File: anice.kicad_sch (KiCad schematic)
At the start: 7 parts, among them J1 Conn_02x20_Counter_Clockwise, J2 Micro_SD_Card_Det1, Y1 ECS-2520MV-xxx-xx

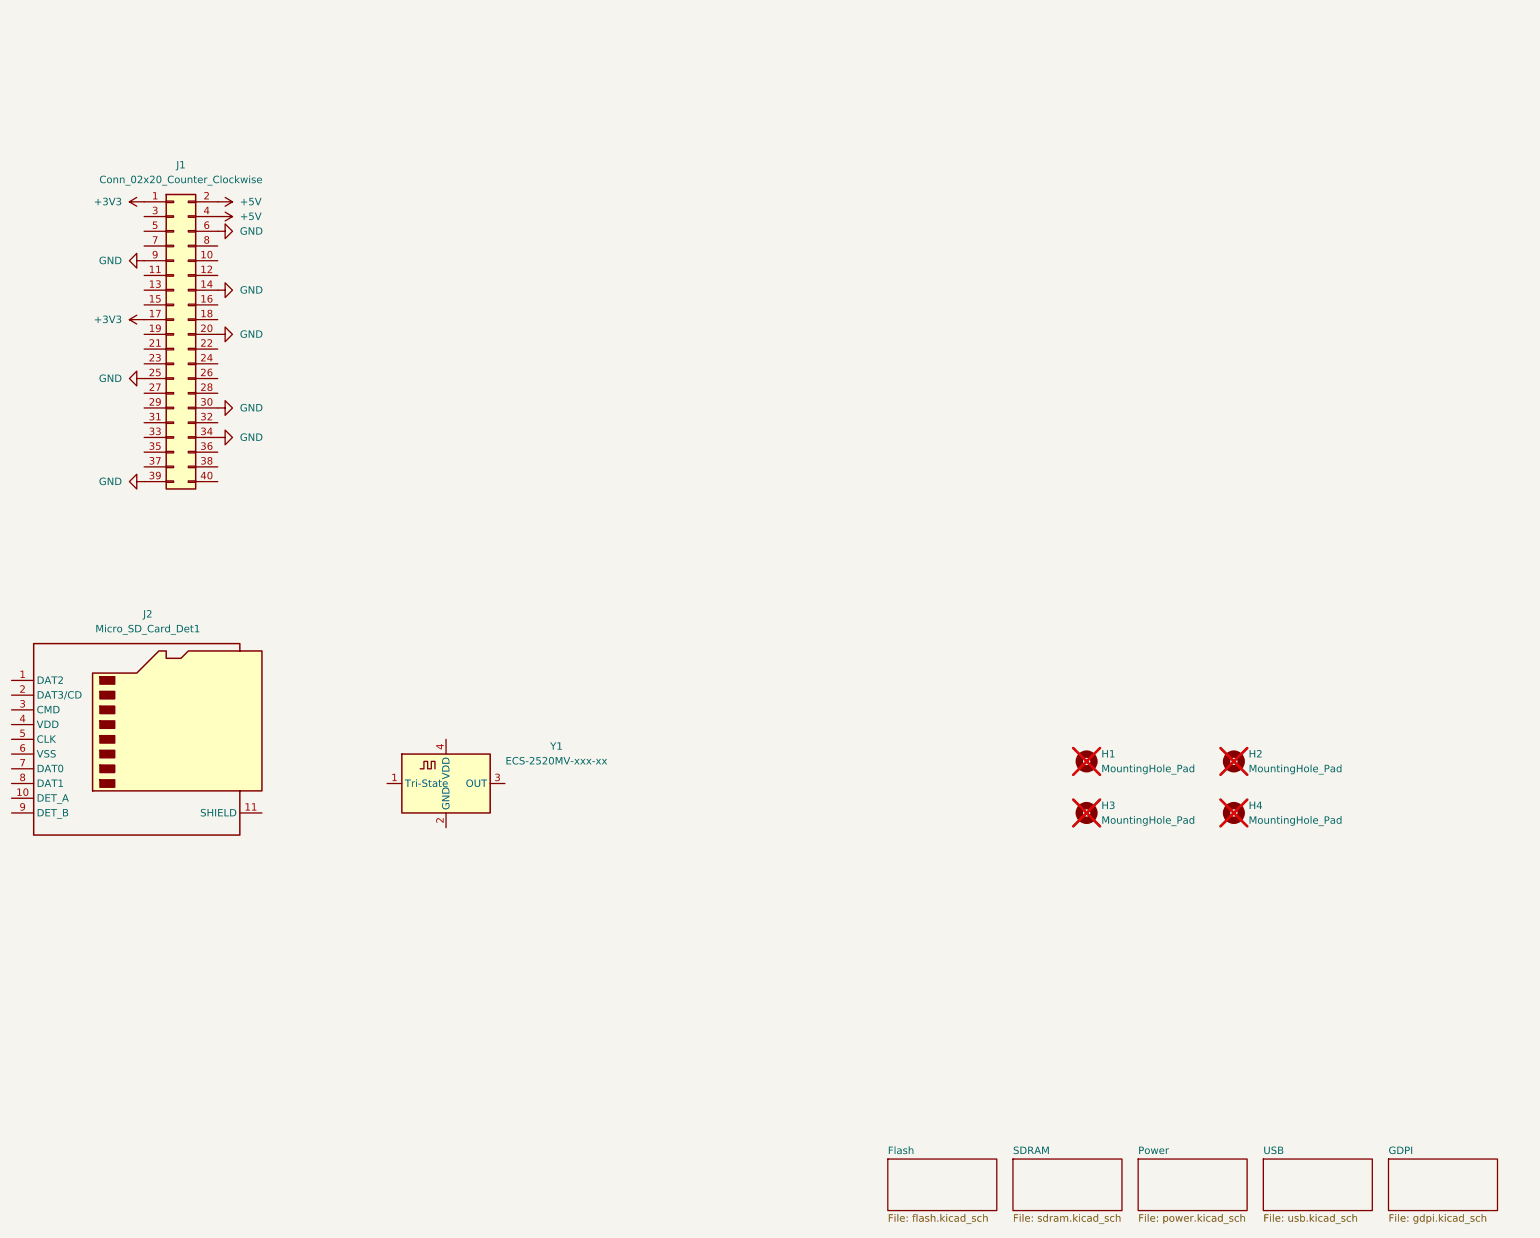
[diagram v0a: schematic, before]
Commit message: Stash
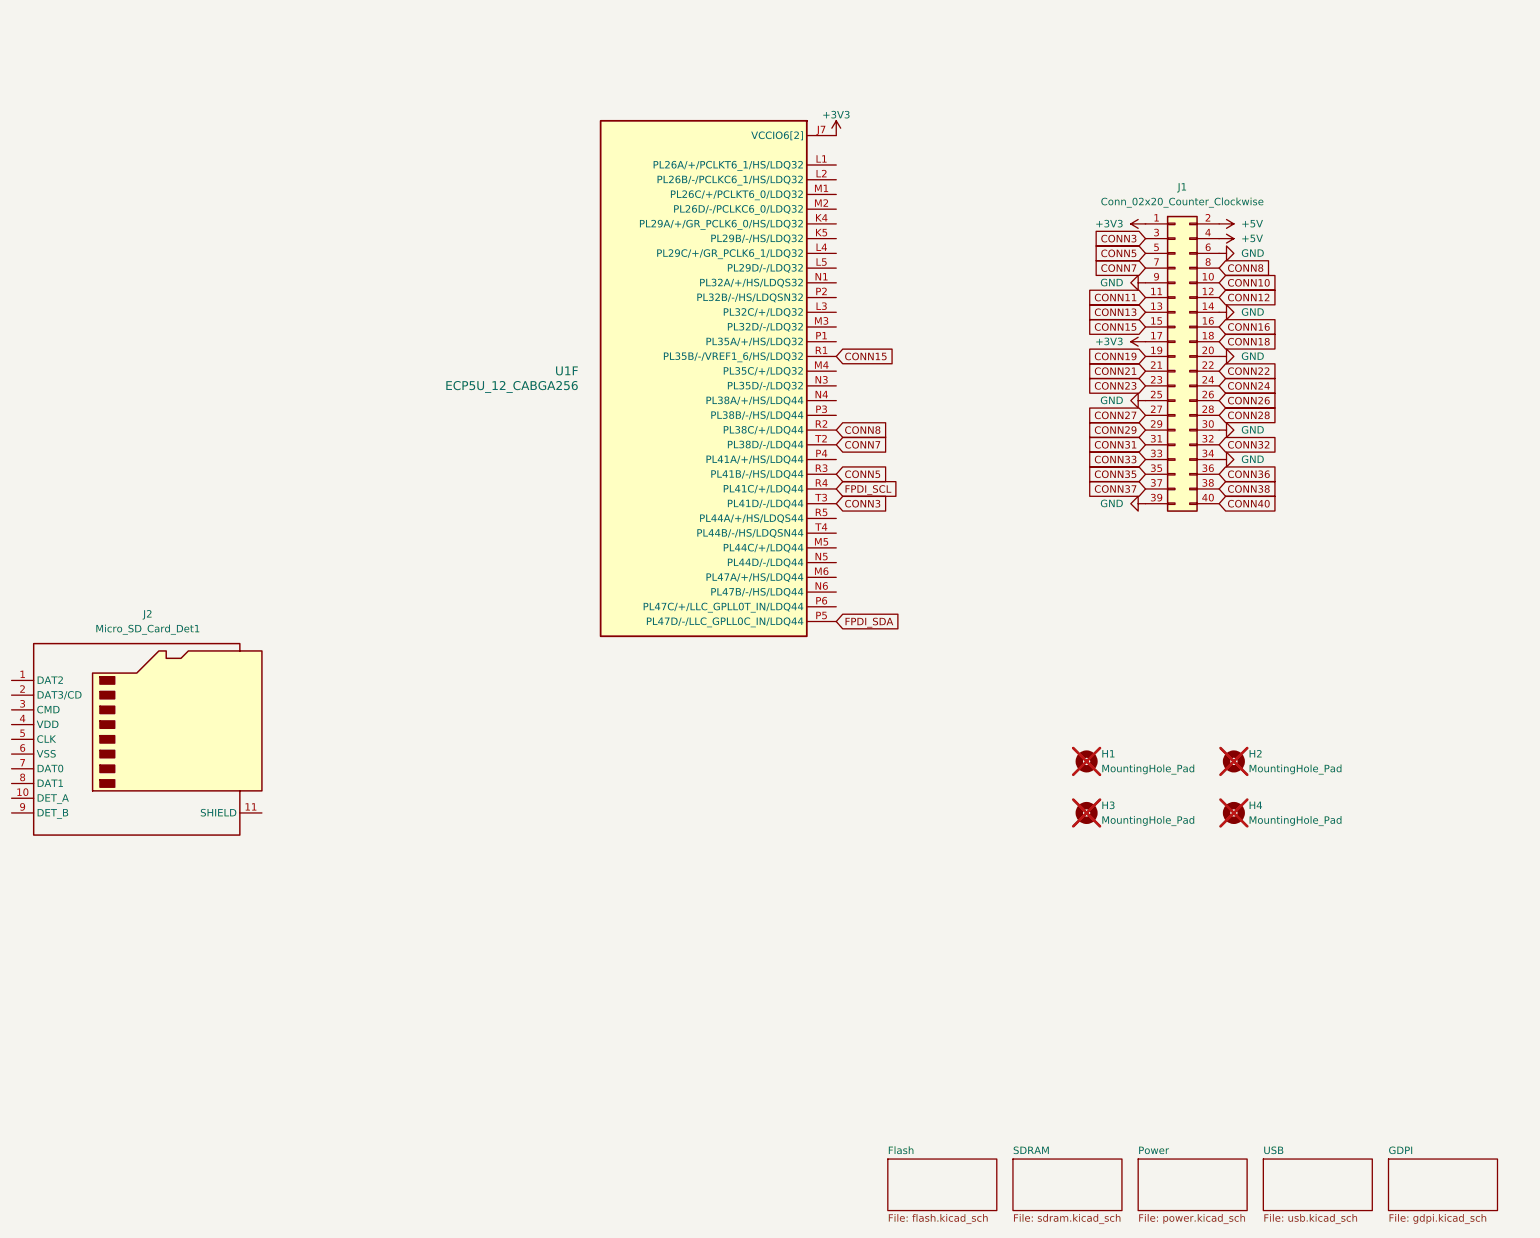
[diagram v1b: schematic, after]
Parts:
- removed Y1: ECS-2520MV-xxx-xx, Crystal:Crystal_SMD_3225-4Pin_3.2x2.5mm, symbol Oscillator:ECS-2520MV-xxx-xx
- added U1: ECP5U_12_CABGA256, Package_BGA:BGA-256_14.0x14.0mm_Layout16x16_P0.8mm_Ball0.45mm_Pad0.32mm_NSMD, symbol josh-ic:ECP5U_12_CABGA256
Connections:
- net +3V3: now also U1.J6 (VCCIO6[2]), U1.J7 (VCCIO6[2])
- net CONN10: now reaches J1.10 (Pin_10)
- net CONN11: now reaches J1.11 (Pin_11)
- net CONN12: now reaches J1.12 (Pin_12)
- net CONN13: now reaches J1.13 (Pin_13)
- net CONN15: now reaches J1.15 (Pin_15)
- net CONN15: now also U1.R1 (PL35B/-/VREF1_6/HS/LDQ32)
- net CONN16: now reaches J1.16 (Pin_16)
- net CONN18: now reaches J1.18 (Pin_18)
- net CONN19: now reaches J1.19 (Pin_19)
- net CONN21: now reaches J1.21 (Pin_21)
- net CONN22: now reaches J1.22 (Pin_22)
- net CONN23: now reaches J1.23 (Pin_23)
- net CONN24: now reaches J1.24 (Pin_24)
- net CONN26: now reaches J1.26 (Pin_26)
- net CONN27: now reaches J1.27 (Pin_27)
- net CONN28: now reaches J1.28 (Pin_28)
- net CONN29: now reaches J1.29 (Pin_29)
- net CONN3: now reaches J1.3 (Pin_3)
- net CONN3: now also U1.T3 (PL41D/-/LDQ44)
- net CONN31: now reaches J1.31 (Pin_31)
- net CONN32: now reaches J1.32 (Pin_32)
- net CONN33: now reaches J1.33 (Pin_33)
- net CONN35: now reaches J1.35 (Pin_35)
- net CONN36: now reaches J1.36 (Pin_36)
- net CONN37: now reaches J1.37 (Pin_37)
- net CONN38: now reaches J1.38 (Pin_38)
- net CONN40: now reaches J1.40 (Pin_40)
- net CONN5: now reaches J1.5 (Pin_5)
- net CONN5: now also U1.R3 (PL41B/-/HS/LDQ44)
- net CONN7: now reaches J1.7 (Pin_7)
- net CONN7: now also U1.T2 (PL38D/-/LDQ44)
- net CONN8: now reaches J1.8 (Pin_8)
- net CONN8: now also U1.R2 (PL38C/+/LDQ44)
- new net FPDI_SCL: U1.R4 (PL41C/+/LDQ44)
- new net FPDI_SDA: U1.P5 (PL47D/-/LLC_GPLL0C_IN/LDQ44)
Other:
- moved on the sheet: J1

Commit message: Rev 1
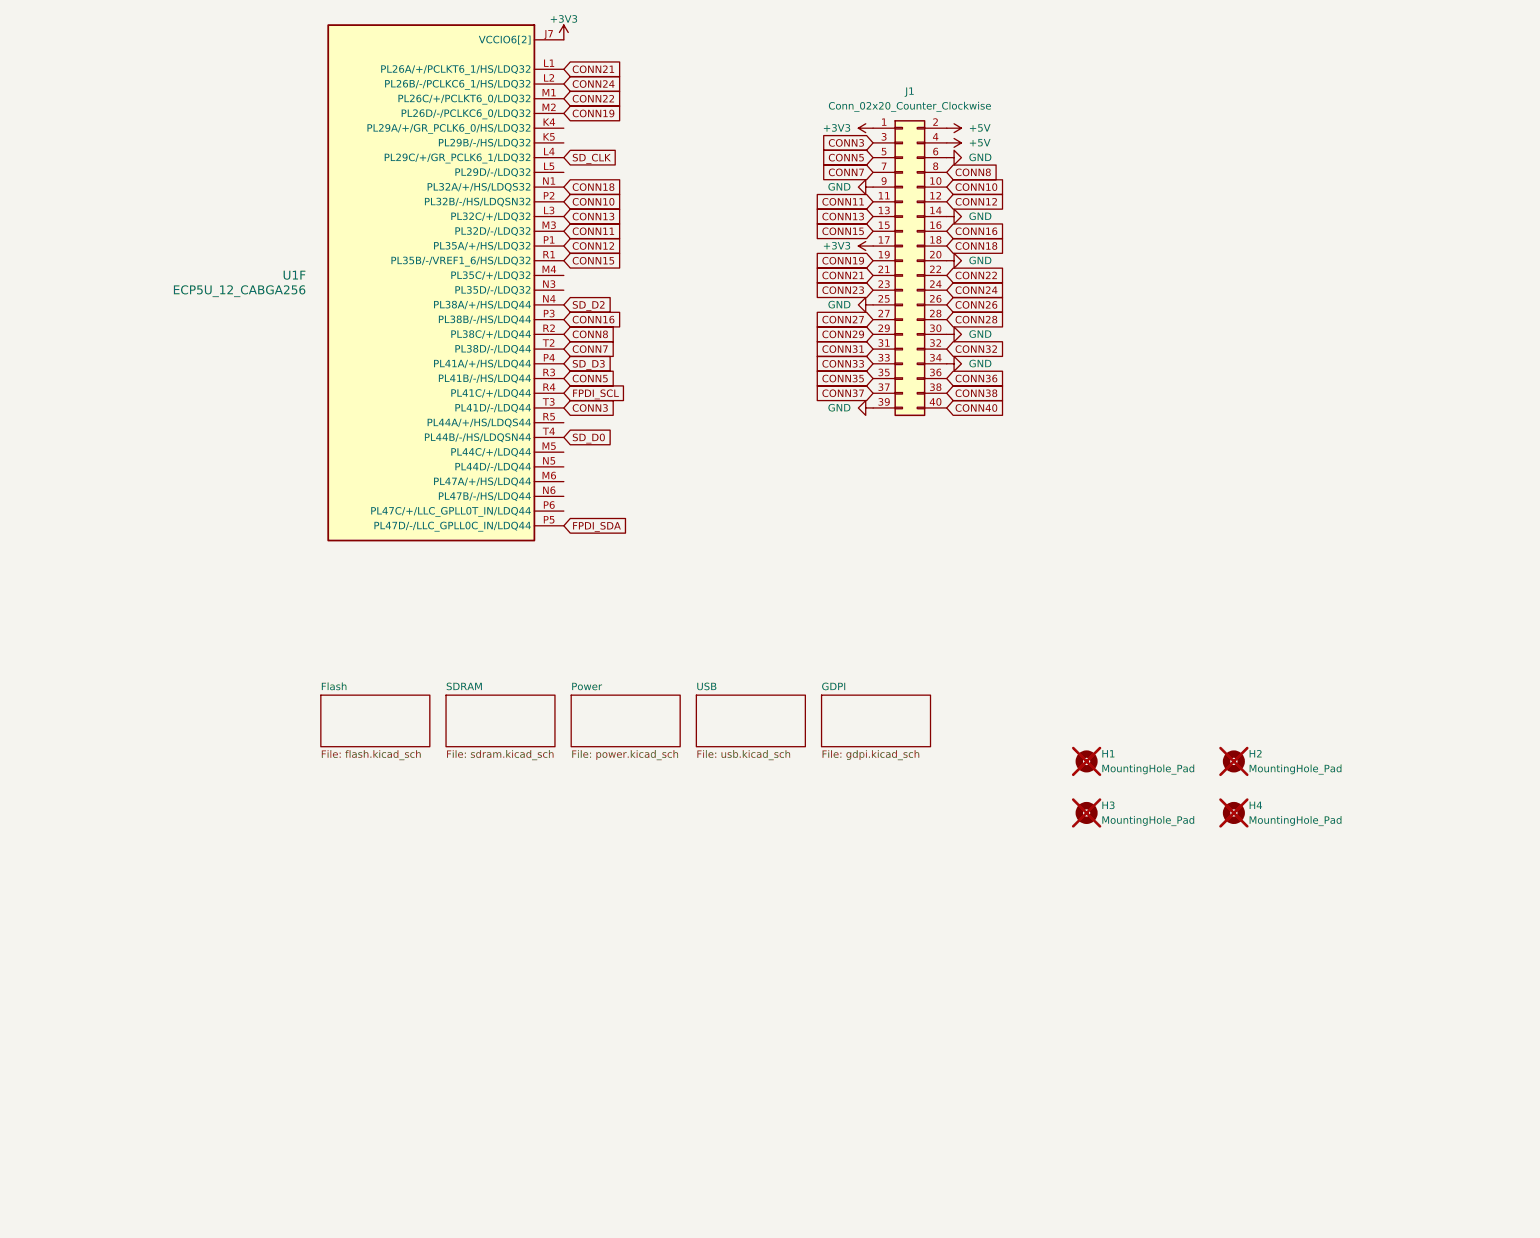
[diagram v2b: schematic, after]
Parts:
- removed J2: Micro_SD_Card_Det1, anice-lib:SDCard molex, symbol Connector:Micro_SD_Card_Det2
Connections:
- net CONN10: now also U1.P2 (PL32B/-/HS/LDQSN32)
- net CONN11: now also U1.M3 (PL32D/-/LDQ32)
- net CONN12: now also U1.P1 (PL35A/+/HS/LDQ32)
- net CONN13: now also U1.L3 (PL32C/+/LDQ32)
- net CONN16: now also U1.P3 (PL38B/-/HS/LDQ44)
- net CONN18: now also U1.N1 (PL32A/+/HS/LDQS32)
- net CONN19: now also U1.M2 (PL26D/-/PCLKC6_0/LDQ32)
- net CONN21: now also U1.L1 (PL26A/+/PCLKT6_1/HS/LDQ32)
- net CONN22: now also U1.M1 (PL26C/+/PCLKT6_0/LDQ32)
- net CONN24: now also U1.L2 (PL26B/-/PCLKC6_1/HS/LDQ32)
- net SD_CLK: now reaches U1.L4 (PL29C/+/GR_PCLK6_1/LDQ32)
- net SD_D2: now reaches U1.N4 (PL38A/+/HS/LDQ44)
- net SD_D3: now reaches U1.P4 (PL41A/+/HS/LDQ44)
- net SD_D0: now reaches U1.T4 (PL44B/-/HS/LDQSN44)
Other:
- moved on the sheet: J1, U1F

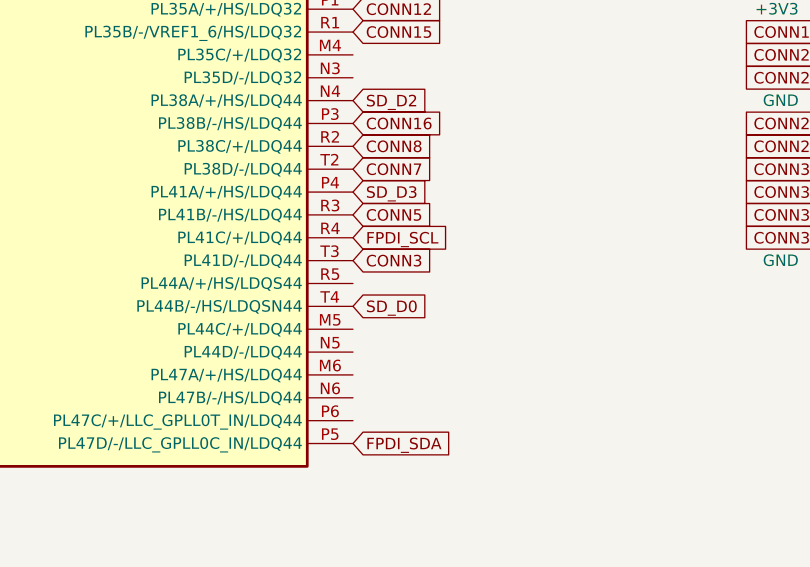
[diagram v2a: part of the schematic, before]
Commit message: No DRC Errors
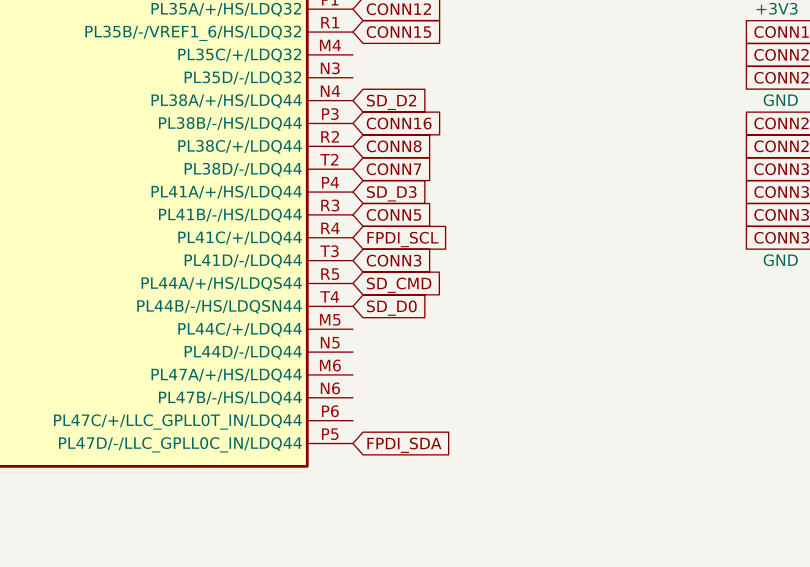
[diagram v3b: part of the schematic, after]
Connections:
- net SD_CMD: now reaches U1.R5 (PL44A/+/HS/LDQS44)
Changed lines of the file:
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@@
+		)
+	)
+	(global_label "SD_CMD"
+		(shape input)
+		(at 137.16 88.9 0)
+		(fields_autoplaced yes)
+		(effects
+			(font
+				(size 1.27 1.27)
+			)
+			(justify left)
+		)
+		(property "Intersheetrefs" "${INTERSHEET_REFS}"
+			(at 147.5837 88.9 0)
+			(effects
+				(font
+					(size 1.27 1.27)
+				)
+				(justify left)
+				(hide yes)
+			)
 		)
 	)
